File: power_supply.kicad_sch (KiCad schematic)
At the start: 18 parts, among them J1 Разъём к автомобилю 2x16 (32 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, U6 MC78M05CDTG, U7 AMS1117-3.3

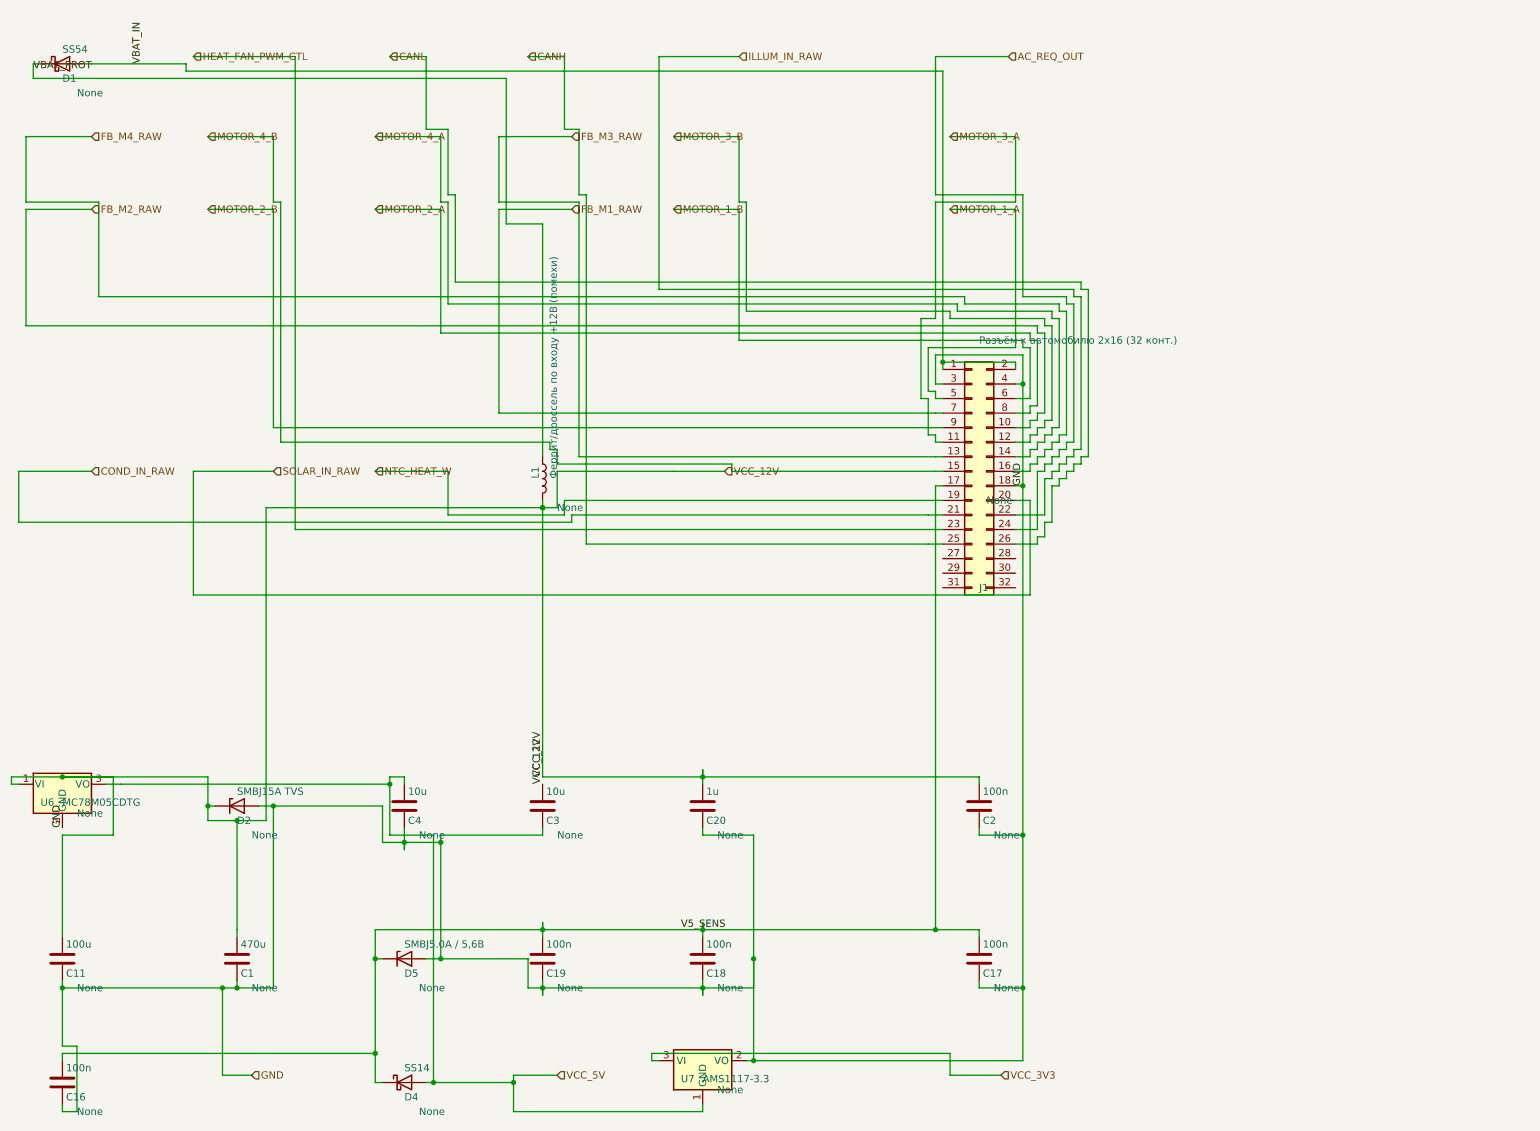
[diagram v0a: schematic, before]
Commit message: tests_fix
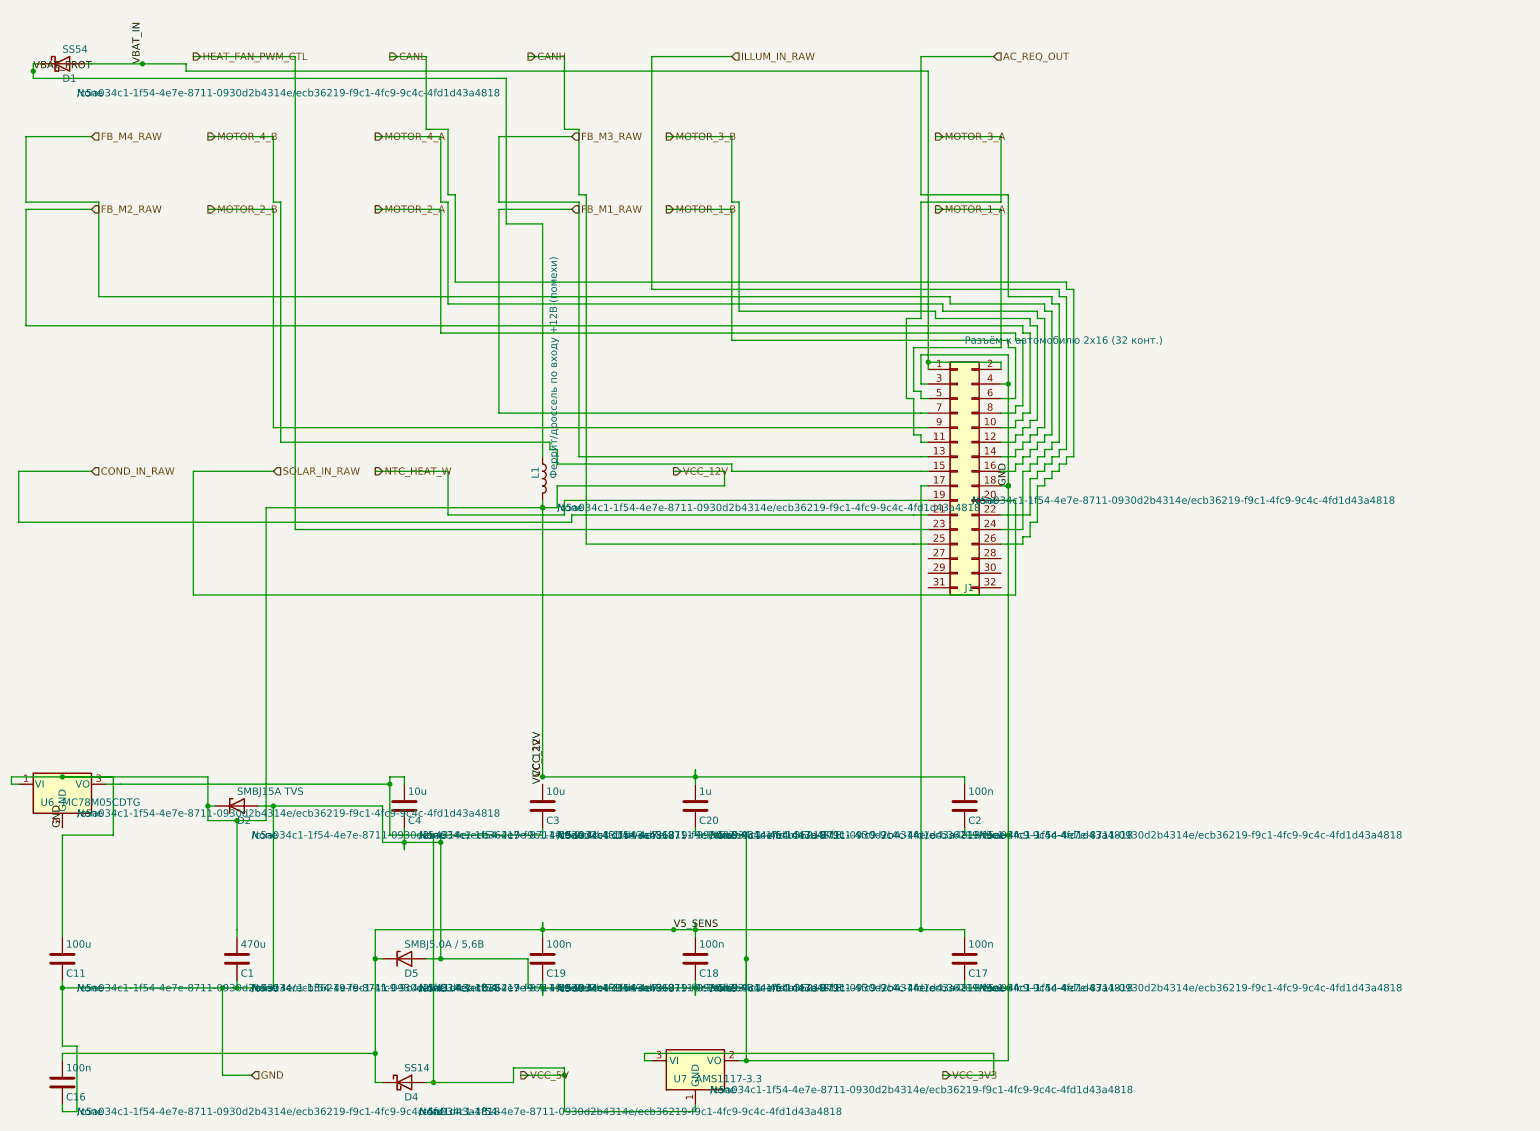
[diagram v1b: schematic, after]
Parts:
- C1, C11, C16, C17, C18, C19, C2, C20, C3, C4, D1, D2, D4, D5, J1, L1, U6, U7: hierarchy_path (none) -> /c5a034c1-1f54-4e7e-8711-0930d2b4314e/ecb36219-f9c1-4fc9-9c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
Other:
- title: (none) -> climate_control_niva_travel

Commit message: refactoring
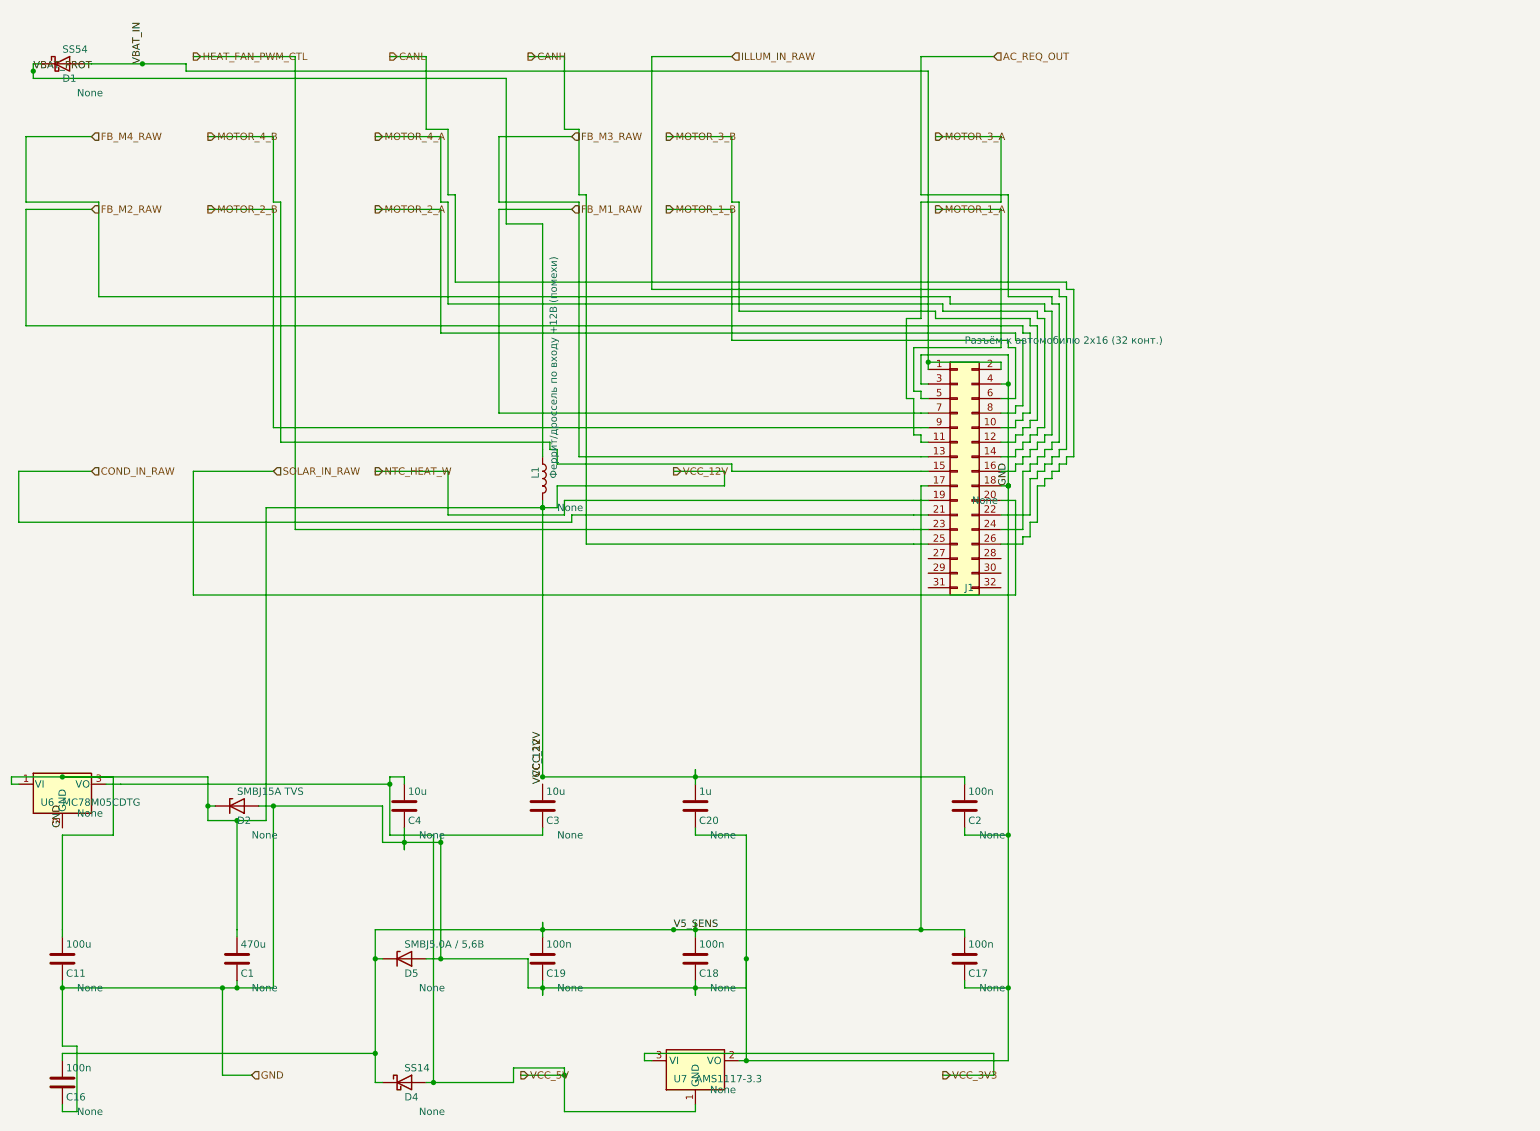
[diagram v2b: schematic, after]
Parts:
- C1, C11, C16, C17, C18, C19, C2, C20, C3, C4, D1, D2, D4, D5, J1, L1, U6, U7: hierarchy_path /c5a034c1-1f54-4e7e-8711-0930d2b4314e/ecb36219-f9c1-4fc9-9c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 -> (none)

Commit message: refactoring
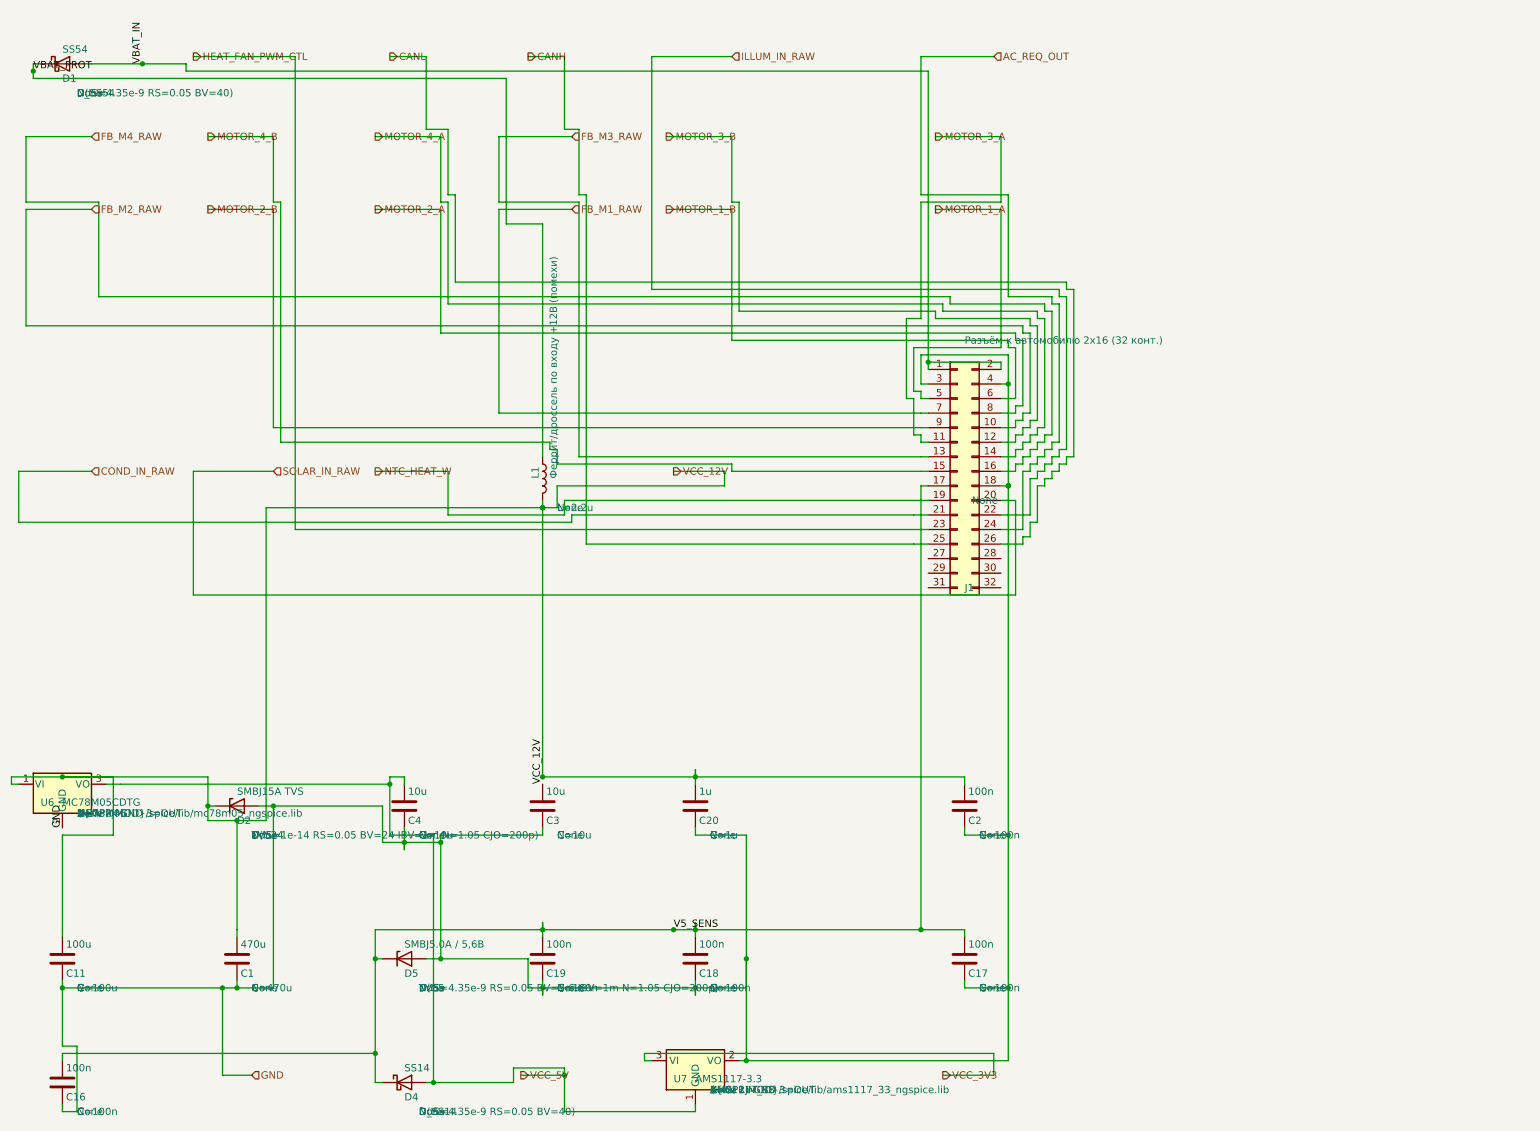
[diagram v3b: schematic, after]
